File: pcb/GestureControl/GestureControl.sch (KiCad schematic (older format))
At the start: 43 parts, among them J1 Conn_01x04_I2I-LCD, J2 BATT, J3 Conn_01x08, J4 Conn_01x06, J5 Conn_01x10, J6 Conn_01x08, SW1 SW1, SW2 SW2, U1 LD1117-3.3, U2 LD1117-5.0

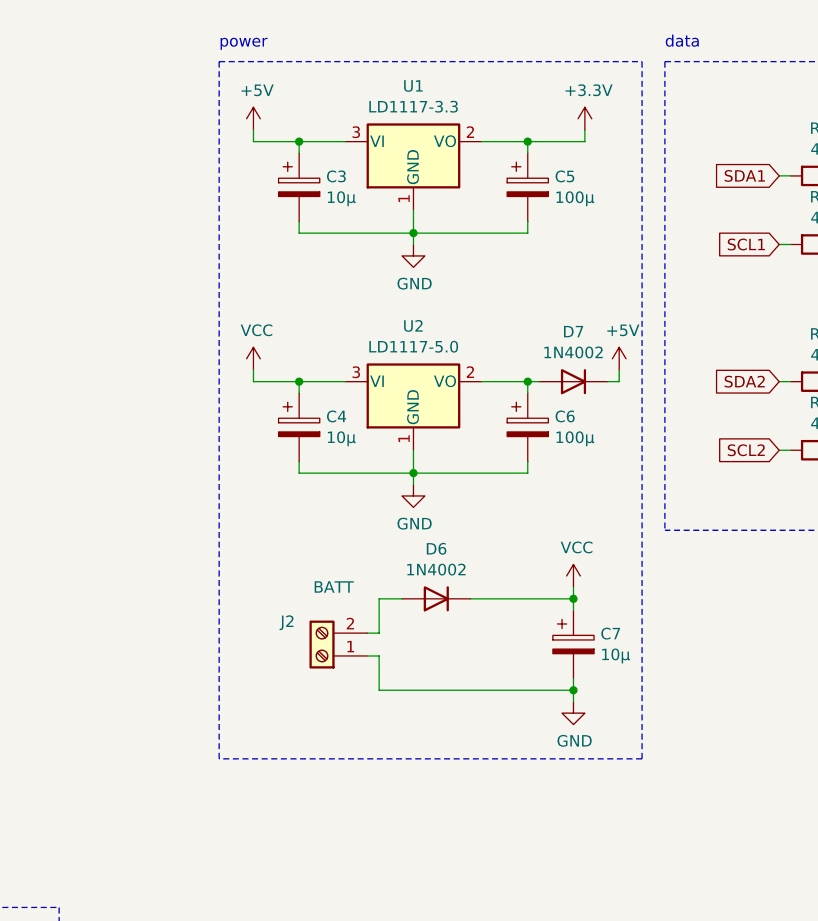
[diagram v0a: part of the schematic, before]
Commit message: add feedback Philip
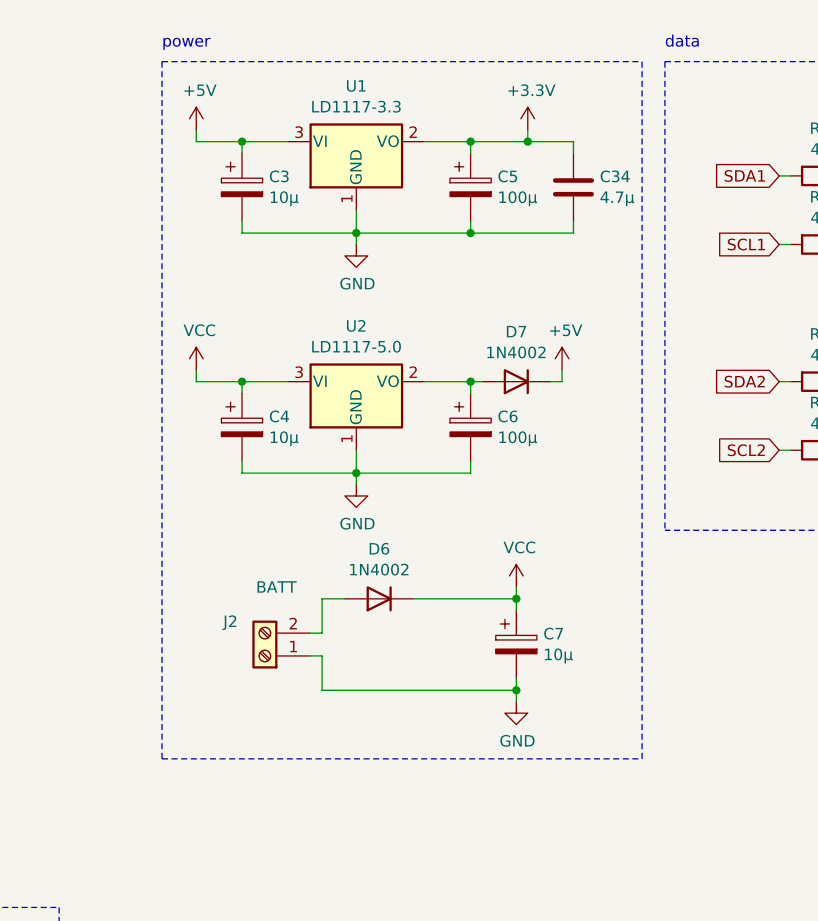
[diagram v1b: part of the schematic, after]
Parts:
- added C34: 4.7µ, Capacitor_SMD:C_0805_2012Metric_Pad1.18x1.45mm_HandSolder, symbol Device:C
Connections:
- net +3V3: now also C34.1
- net GND: now also C34.2
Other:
- moved on the sheet: C3, C4, C5, C6, C7, D6, D7, J2, U1, U2

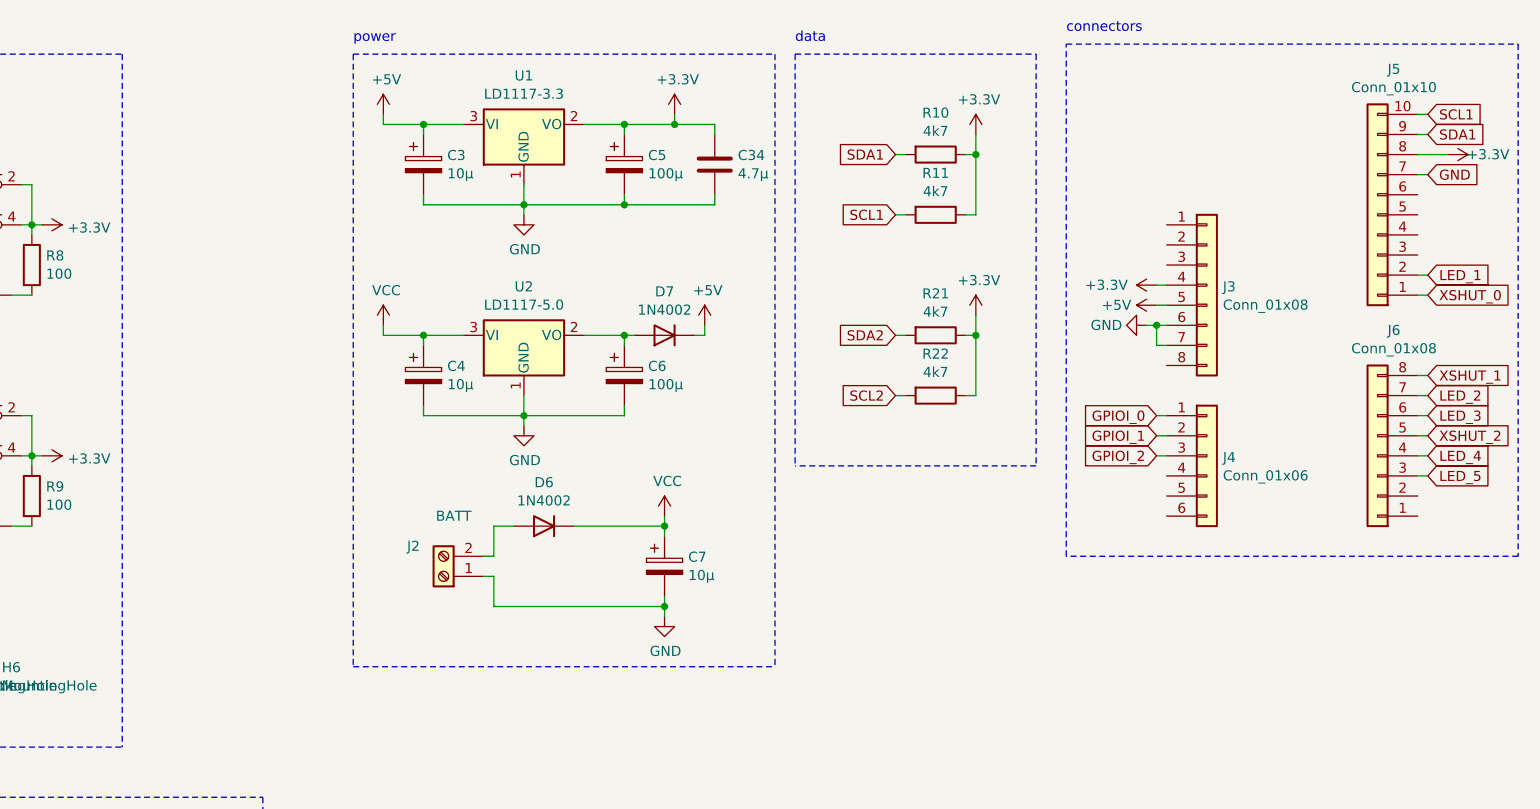
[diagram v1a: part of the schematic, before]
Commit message: werking printf()
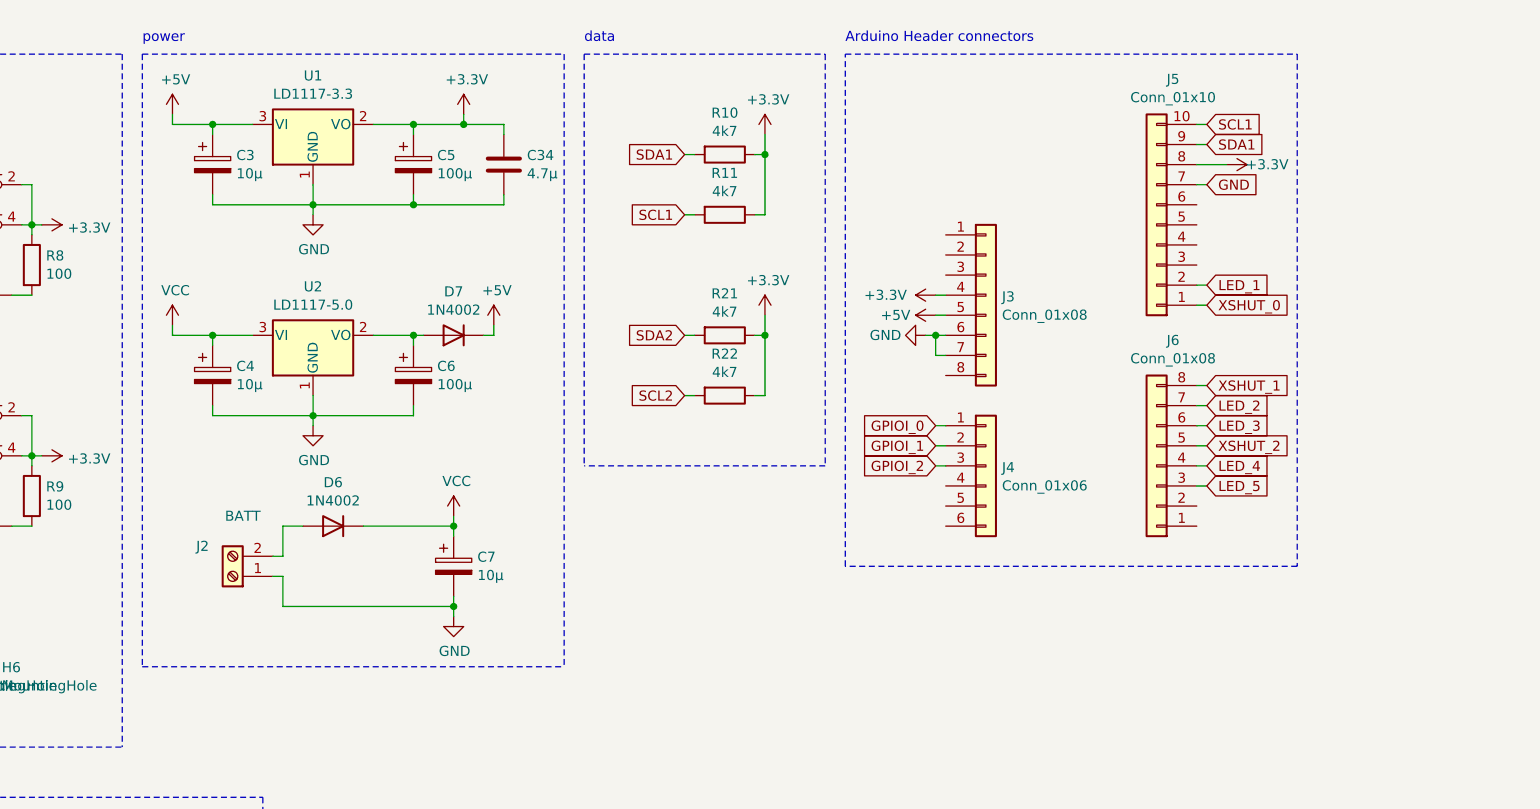
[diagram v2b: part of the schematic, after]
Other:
- note added: "Arduino Header connectors"
- note removed: "connectors"
- moved on the sheet: C3, C34, C4, C5, C6, C7, D6, D7, J2, J3, J4, J5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

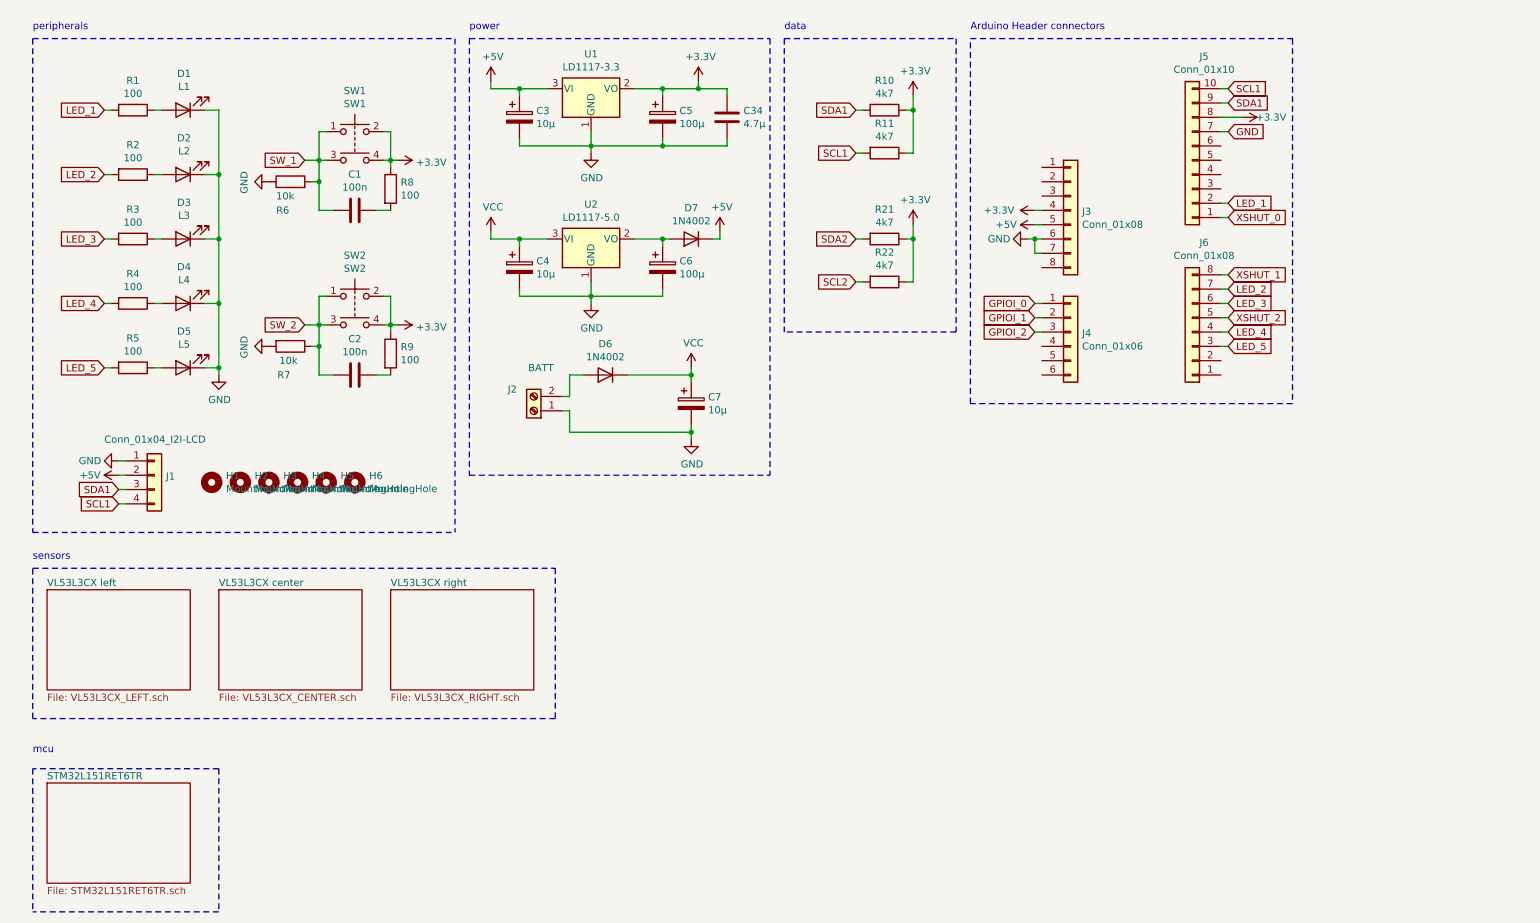
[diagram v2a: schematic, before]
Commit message: add PCBV0.11
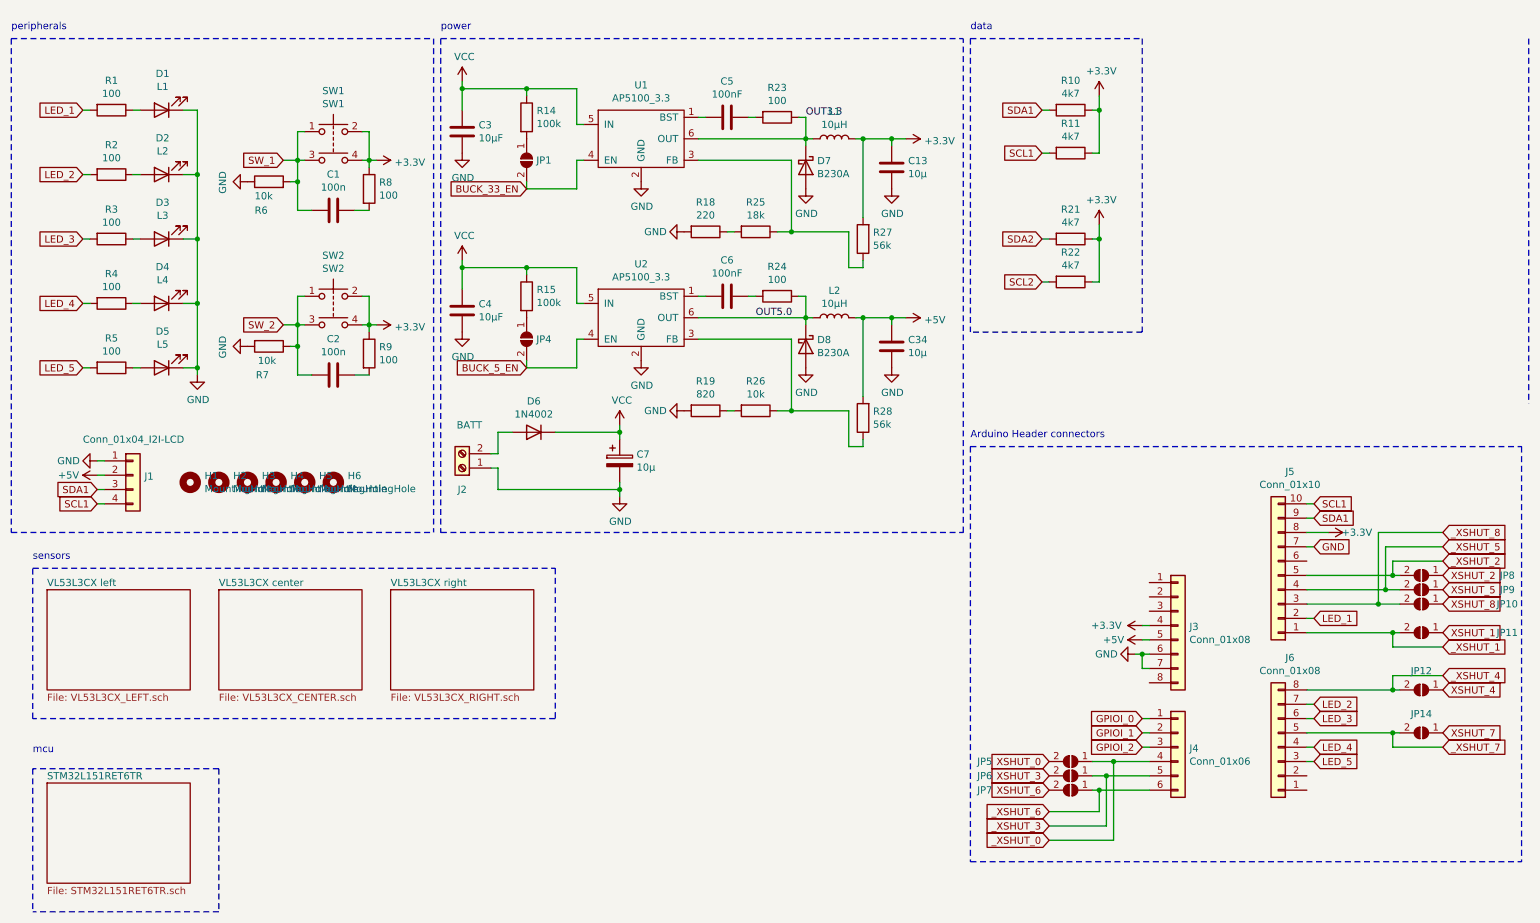
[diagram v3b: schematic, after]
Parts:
- removed C3, C4: 10µ, Capacitor_SMD:CP_Elec_6.3x5.4, symbol Device:CP
- removed C5, C6: 100µ, Capacitor_SMD:CP_Elec_6.3x5.4, symbol Device:CP
- removed D7: 1N4002, Diode_SMD:D_SMA_Handsoldering, symbol Device:D
- removed U1: LD1117-3.3, Package_TO_SOT_SMD:SOT-223-3_TabPin2, symbol Regulator_Linear:AMS1117-3.3
- removed U2: LD1117-5.0, Package_TO_SOT_SMD:SOT-223-3_TabPin2, symbol Regulator_Linear:AMS1117-5.0
- added C13: 10µ, Capacitor_SMD:C_1206_3216Metric_Pad1.33x1.80mm_HandSolder, symbol Device:C
- added C3, C4: 10µF, Capacitor_SMD:C_1206_3216Metric_Pad1.33x1.80mm_HandSolder, symbol Device:C
- added C5, C6: 100nF, Capacitor_SMD:C_0603_1608Metric_Pad1.08x0.95mm_HandSolder, symbol Device:C
- added D7, D8: B230A, Diode_SMD:D_SMA_Handsoldering, symbol Device:D_Schottky
- added JP1, JP10, JP11, JP12, JP14, JP4, JP5, JP6, JP7, JP8, JP9: SolderJumper_2_Open, Jumper:SolderJumper-2_P1.3mm_Open_Pad1.0x1.5mm, symbol Jumper:SolderJumper_2_Open
- added L1, L2: 10µH, Inductor_SMD:L_Taiyo-Yuden_NR-50xx_HandSoldering, symbol Device:L
- added R14, R15: 100k, Resistor_SMD:R_0805_2012Metric_Pad1.20x1.40mm_HandSolder, symbol Device:R
- added R18: 220, Resistor_SMD:R_0805_2012Metric_Pad1.20x1.40mm_HandSolder, symbol Device:R
- added R19: 820, Resistor_SMD:R_0805_2012Metric_Pad1.20x1.40mm_HandSolder, symbol Device:R
- added R23, R24: 100, Resistor_SMD:R_0805_2012Metric_Pad1.20x1.40mm_HandSolder, symbol Device:R
- added R25: 18k, Resistor_SMD:R_0805_2012Metric_Pad1.20x1.40mm_HandSolder, symbol Device:R
- added R26: 10k, Resistor_SMD:R_0805_2012Metric_Pad1.20x1.40mm_HandSolder, symbol Device:R
- added R27, R28: 56k, Resistor_SMD:R_0805_2012Metric_Pad1.20x1.40mm_HandSolder, symbol Device:R
- added U1, U2: AP5100_3.3, Package_TO_SOT_SMD:TSOT-23-6_HandSoldering, symbol AP5100:AP5100
- C34: value 4.7µ -> 10µ; footprint Capacitor_SMD:C_0805_2012Metric_Pad1.18x1.45mm_HandSolder -> Capacitor_SMD:C_1206_3216Metric_Pad1.33x1.80mm_HandSolder
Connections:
- net +3V3: now also C13.1, L1.2, R27.2; no longer C34.1
- net +5V: now also C34.1, L2.2, R28.2
- net GND: now also C13.2, C3.2, C4.2, D7.2 (A), D8.2 (A), R18.2, R19.2, U1.2 (GND), U2.2 (GND)
- net VCC: now also C3.1, C4.1, R14.1, R15.1, U1.5 (IN), U2.5 (IN)
- net XSHUT_0: now also JP5.2 (B); no longer J5.1 (Pin_1)
- net XSHUT_1: now also JP11.1 (A); no longer J6.8 (Pin_8)
- net XSHUT_2: now also JP8.1 (A); no longer J6.5 (Pin_5)
- net _XSHUT_0: now reaches J4.4 (Pin_4)
- net _XSHUT_0: now also JP5.1 (A)
- net _XSHUT_3: now reaches J4.5 (Pin_5)
- net _XSHUT_3: now also JP6.1 (A)
- net _XSHUT_6: now reaches J4.6 (Pin_6)
- net _XSHUT_6: now also JP7.1 (A)
- net _XSHUT_8: now reaches J5.3 (Pin_3)
- net _XSHUT_8: now also JP10.2 (B)
- net _XSHUT_5: now reaches J5.4 (Pin_4)
- net _XSHUT_5: now also JP9.2 (B)
- net _XSHUT_2: now reaches J5.5 (Pin_5)
- net _XSHUT_2: now also JP8.2 (B)
- new net: C5.2, U1.1 (BST)
- new net: R25.1, R27.1, U1.3 (FB)
- new net: JP1.1 (A), R14.2
- new net: C5.1, R23.2
- new net: R18.1, R25.2
- new net: C6.2, U2.1 (BST)
- new net: R26.1, R28.1, U2.3 (FB)
- new net: JP4.1 (A), R15.2
- new net: C6.1, R24.2
- new net: R19.1, R26.2
- new net BUCK_33_EN: JP1.2 (B), U1.4 (EN)
- new net BUCK_5_EN: JP4.2 (B), U2.4 (EN)
- new net OUT3.3: D7.1 (K), L1.1, R23.1, U1.6 (OUT)
- new net OUT5.0: D8.1 (K), L2.1, R24.1, U2.6 (OUT)
- new net XSHUT_3: JP6.2 (B)
- new net XSHUT_4: JP12.1 (A)
- new net XSHUT_5: JP9.1 (A)
- new net XSHUT_6: JP7.2 (B)
- new net XSHUT_7: JP14.1 (A)
- new net XSHUT_8: JP10.1 (A)
- new net _XSHUT_1: J5.1 (Pin_1), JP11.2 (B)
- new net _XSHUT_4: J6.8 (Pin_8), JP12.2 (B)
- new net _XSHUT_7: J6.5 (Pin_5), JP14.2 (B)
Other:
- moved on the sheet: C1, C2, C7, D1, D2, D3, D4, D5, D6, H1, H2, H3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
